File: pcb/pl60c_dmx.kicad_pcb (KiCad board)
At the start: 2 copper layers, 80 x 54 mm, 39 parts, among them J1 USB-C 16P, J2 XLR-5 female (DMX OUT), J3 DMX pigtail, J4 EXPANSION, J5 UART0, Q1 S8050, SW1 RESET, SW2 BOOT, SW3 USER, U1 ESP32-S3-WROOM-1-N16R8, U2 AMS1117-3.3, U3 SP3485EN, U4 USBLC6-2SC6

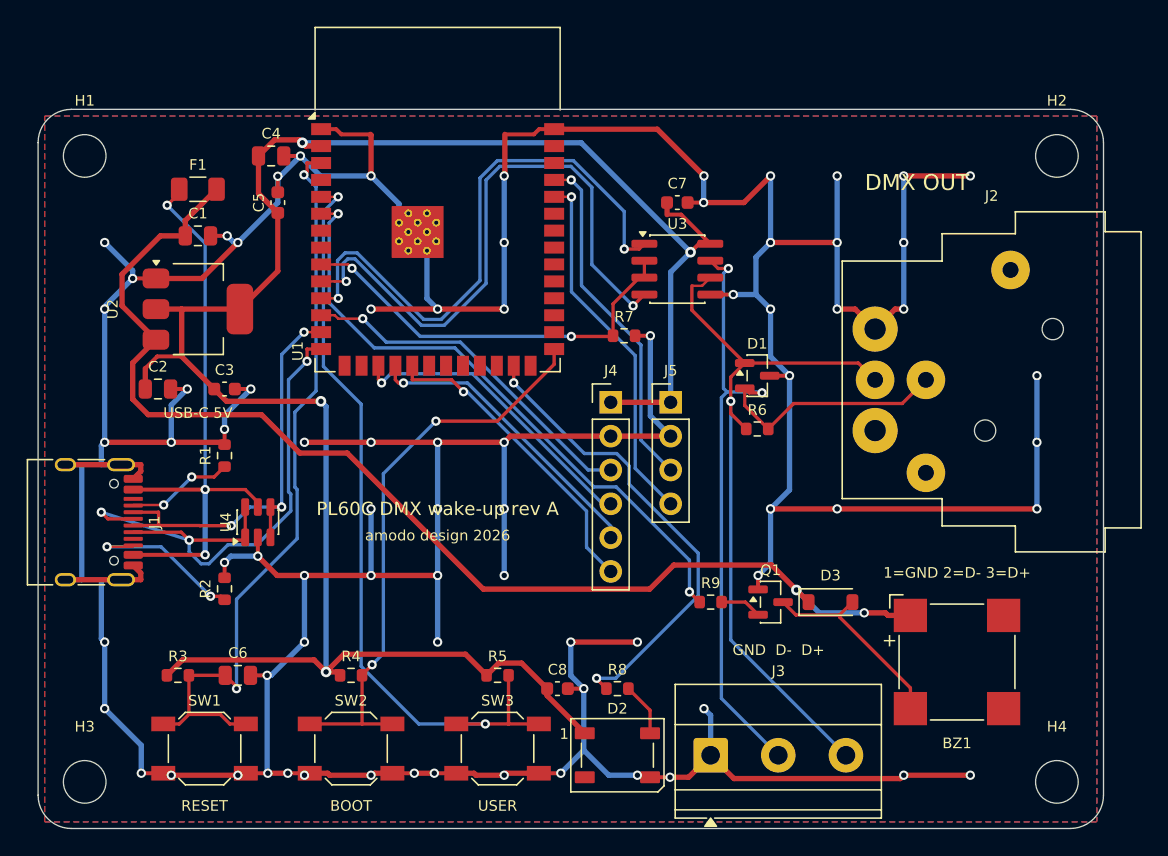
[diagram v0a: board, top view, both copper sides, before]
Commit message: auto: 2026-09-02 13:27:07
Co-Authored-By: Claude Fable 5.1 <noreply@anthropic.com>
Claude-Session: https://claude.ai/code/session_01WsrVZb94LwbHVAmBvsSTfn
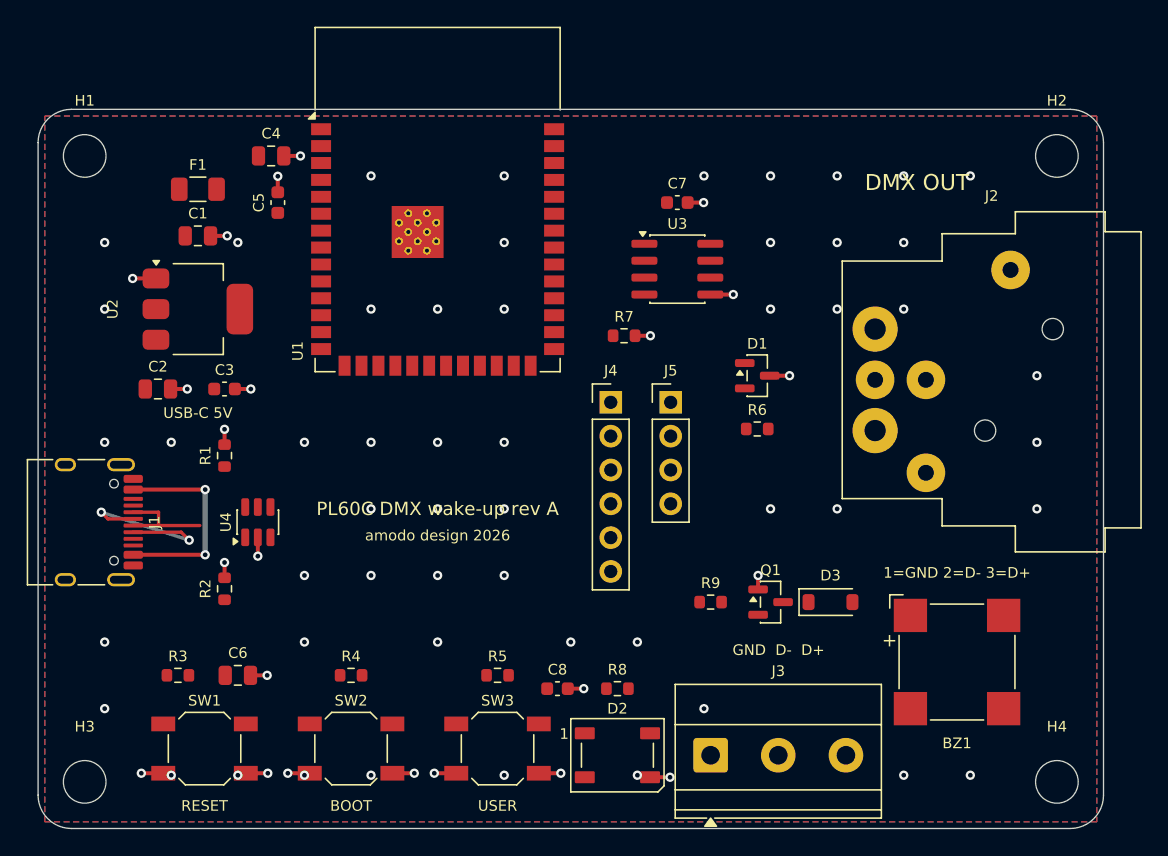
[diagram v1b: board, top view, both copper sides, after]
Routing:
- net GND: track 480.5 -> 32.1 mm
- net +3V3: track 158.8 -> 0.00 mm, vias 4 -> 0
- net +5V: track 89.5 -> 0.00 mm, vias 2 -> 0
- net DMX_B: track 61.6 -> 0.00 mm, vias 2 -> 0
- net BTN_USER: track 59.1 -> 0.00 mm, vias 2 -> 0
- net EN: track 57.4 -> 0.00 mm, vias 2 -> 0
- net DMX_A: track 55.4 -> 0.00 mm, vias 1 -> 0
- net BUZZER: track 46.8 -> 0.00 mm, vias 2 -> 0
- net DMX_TX: track 45.7 -> 0.00 mm, vias 2 -> 0
- net DMX_RX: track 43.5 -> 0.00 mm, vias 2 -> 0
- net IO0_BOOT: track 43.0 -> 0.00 mm, vias 2 -> 0
- net LED_DATA: track 35.7 -> 0.00 mm, vias 2 -> 0
- net DMX_DE: track 31.0 -> 0.00 mm, vias 2 -> 0
- net USB_D+: track 44.9 -> 14.0 mm, vias 3 -> 2
- net VBUS: track 44.5 -> 15.7 mm, vias 3 -> 2
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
